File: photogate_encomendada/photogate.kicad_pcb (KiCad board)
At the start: 2 copper layers, 77.9 x 64.8 mm, 23 parts, among them P2 3poles LOGO

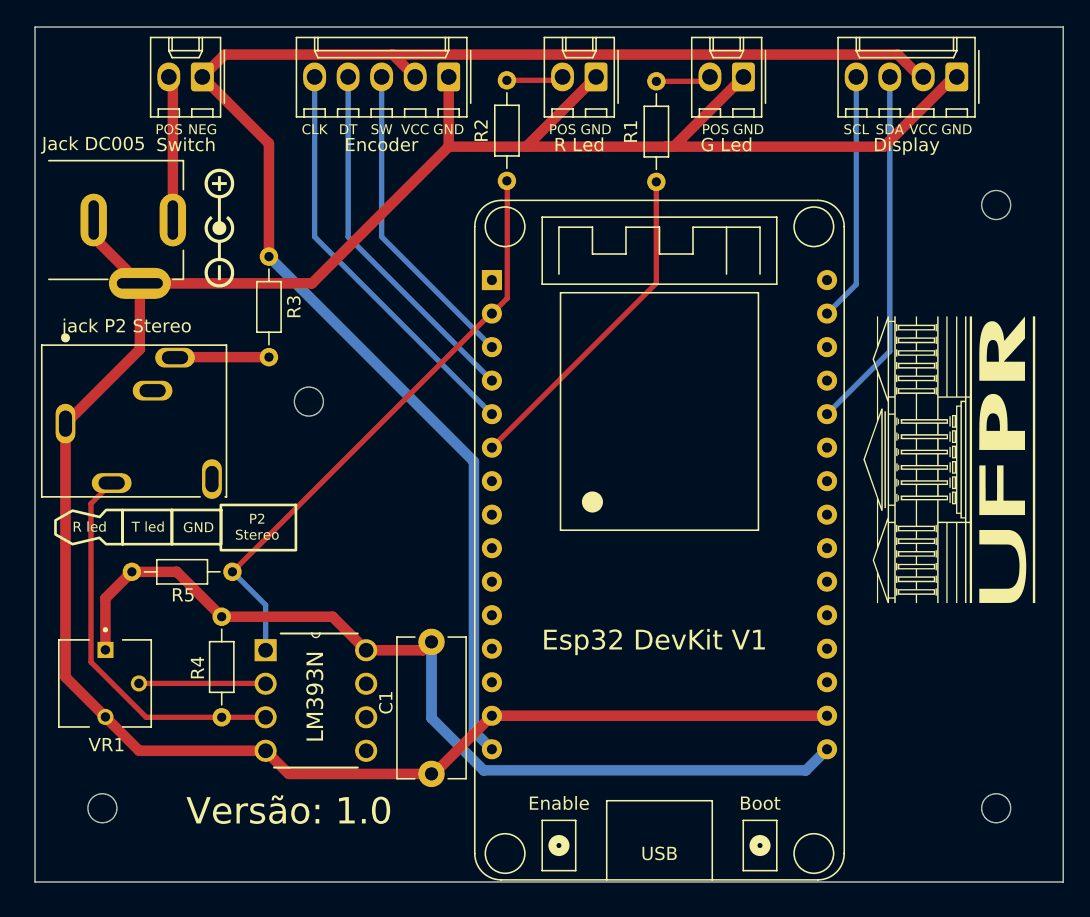
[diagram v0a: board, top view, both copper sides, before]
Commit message: Placas de fenolite e perfurada acabadas
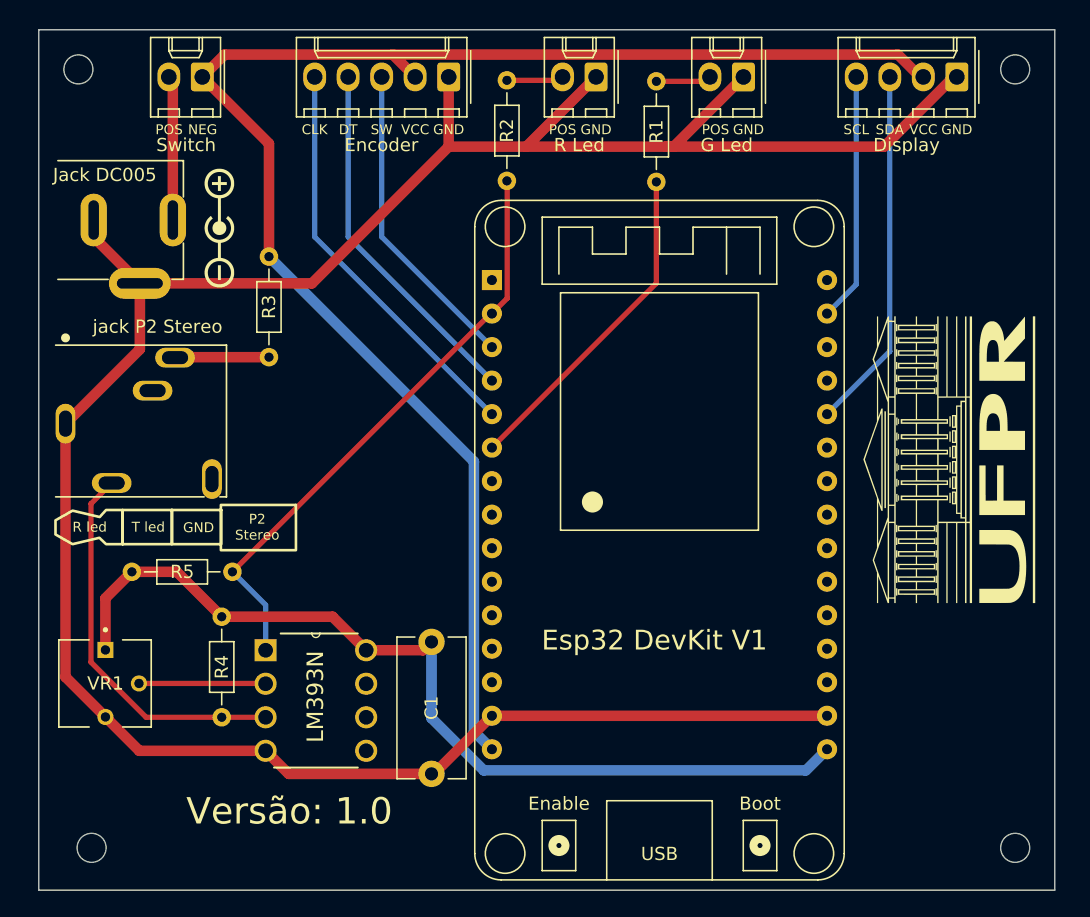
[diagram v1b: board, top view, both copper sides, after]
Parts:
- moved Furo Central 30.6 mm to (93.0, 71.0)
- moved Furo Superior 10.4 mm to (164.0, 71.0)
- moved Furo Inferior2 3.33 mm to (164.0, 130.0)
- moved Furo Inferior1 3.11 mm to (94.0, 130.0)
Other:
- board size 77.9 x 64.8 mm -> 77 x 65.2 mm
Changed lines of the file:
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@@
     (property "Sheetname" "")
     (attr through_hole)
-    (fp_text reference "jack P2 Stereo" (at 4.651 -7.3875 180) (layer "F.SilkS")
+    (fp_text reference "jack P2 Stereo" (at 6.9772 -7.3509) (layer "F.SilkS")
       (effects (font (size 1 1) (thickness 0.15)))
     )
@@
       (effects (font (size 1.401937 1.401937) (thickness 0.15)))
     )
-    (fp_line (start 10.2 5.55) (end -1.8 5.55) (layer "F.SilkS") (width 0.127))
-    (fp_line (start -1.8 5.55) (end -1.8 -5.95) (layer "F.SilkS") (width 0.127))
-    (fp_line (start -1.8 -5.95) (end 12.2 -5.95) (layer "F.SilkS") (width 0.127))
-    (fp_line (start 12.2 5.55) (end 12.1 5.55) (layer "F.SilkS") (width 0.127))
+    (fp_line (start -0.75 -5.95) (end 12.2 -5.95) (layer "F.SilkS") (width 0.127))
+    (fp_line (start 12.2 5.55) (end 11.7 5.55) (layer "F.SilkS") (width 0.127))
+    (fp_line (start -0.75 5.55) (end 10.5 5.55) (layer "F.SilkS") (width 0.127))
     (fp_line (start 12.2 -5.95) (end 12.2 5.55) (layer "F.SilkS") (width 0.127))
     (fp_circle (center 0 -6.5) (end 0.17 -6.5) (layer "F.SilkS") (width 0.34) (fill none))
@@
     (fp_line (start -5.6 3.3) (end -2.1 3.3) (layer "F.CrtYd") (width 0.05))
     (fp_line (start -5.6 -3.3) (end -5.6 3.3) (layer "F.CrtYd") (width 0.05))
-    (fp_line (start -1.8 -5.95) (end -1.8 -3) (layer "F.Fab") (width 0.127))
+    (fp_line (start -1.8 5.55) (end -1.8 -5.95) (layer "F.Fab") (width 0.127))
     (fp_line (start -5.3 -3) (end -5.3 3) (layer "F.Fab") (width 0.127))
     (fp_line (start -1.8 -3) (end -5.3 -3) (layer "F.Fab") (width 0.127))
@@
     (pad "5" thru_hole oval (at 6.6 -2.5) (size 3.016 1.508) (drill oval 2 1) (layers *.Cu *.Mask)
       (net 32 "unconnected-(P2jack1-Pad5)") (pintype "passive"))
-    (model "/home/cold/.local/share/kicad/6.0/footprints/MyFootprints.pretty/CUI_DEVICES_SJ1-3515N.step"
+    (model "/home/cold/.local/share/kicad/6.0/footprints/MyJacks.pretty/CUI_DEVICES_SJ1-3515N.step"
       (offset (xyz -5.3 0 2.5))
       (scale (xyz 1 1 1))
@@
     (property "Sheetname" "")
     (attr through_hole)
-    (fp_text reference "VR1" (at 4.6736 -0.1016 180) (layer "F.SilkS")
+    (fp_text reference "VR1" (at 0 0 180) (layer "F.SilkS")
       (effects (font (size 1.002756 1.002756) (thickness 0.15)))
     )
@@
     (pad "3" thru_hole circle (at 2.54 0 270) (size 1.222 1.222) (drill 0.714) (layers *.Cu *.Mask)
       (net 2 "GND") (pintype "passive"))
-    (model "/home/cold/.local/share/kicad/6.0/footprints/MyFootprints.pretty/TRIM_3362P-1-103.step"
+    (model "/home/cold/.local/share/kicad/6.0/footprints/trimpot.pretty/3362P-1-102.STEP"
       (offset (xyz 0 0 0))
       (scale (xyz 1 1 1))
@@
       )
     )
-    (model "/home/cold/.local/share/kicad/6.0/footprints/MyFootprints.pretty/LM393N.step"
+    (model "/home/cold/.local/share/kicad/6.0/footprints/MyCIs.pretty/LM393P.STEP"
       (offset (xyz 0 0.69 -0.5))
       (scale (xyz 1 1 1))
@@
   )
   (footprint "MountingHole:MountingHole_2.2mm_M2" (layer "F.Cu")
-    (at 162.56 127)
+    (at 164 130)
     (descr "Mounting Hole 2.2mm, no annular, M2")
     (tags "mounting hole 2.2mm no annular m2")
@@
     (property "Sheetname" "")
     (attr through_hole)
-    (fp_text reference "R5" (at 3.7338 -1.778) (layer "F.SilkS")
+    (fp_text reference "R5" (at 3.81 0) (layer "F.SilkS")
       (effects (font (size 1 1) (thickness 0.15)))
     )
@@
     (property "Sheetname" "")
     (attr through_hole)
-    (fp_text reference "Jack DC005" (at -2.29 -5.7612) (layer "F.SilkS")
+    (fp_text reference "Jack DC005" (at -1.4478 -3.4184) (layer "F.SilkS")
       (effects (font (size 1 1) (thickness 0.15)))
     )
@@
       (effects (font (size 0 0) (thickness 0.15)))
     )
-    (fp_line (start 4.51 2.3) (end 4.51 4.5) (layer "F.SilkS") (width 0.127))
-    (fp_line (start -5.6896 -4.5) (end 4.51 -4.5) (layer "F.SilkS") (width 0.127))
-    (fp_line (start 4.51 4.5) (end 3.71 4.5) (layer "F.SilkS") (width 0.127))
-    (fp_line (start -1.2192 4.5) (end -5.6896 4.5) (layer "F.SilkS") (width 0.127))
-    (fp_line (start 4.51 -4.5) (end 4.51 -2.3) (layer "F.SilkS") (width 0.127))
+    (fp_line (start 4.51 1.75) (end 4.51 4.5) (layer "F.SilkS") (width 0.127))
+    (fp_line (start 3.65 4.5) (end 4.51 4.5) (layer "F.SilkS") (width 0.127))
+    (fp_line (start -5 -4.5) (end 4.51 -4.5) (layer "F.SilkS") (width 0.127))
+    (fp_line (start -5 4.5) (end -1.2 4.5) (layer "F.SilkS") (width 0.127))
+    (fp_line (start 4.51 -4.5) (end 4.51 -1.75) (layer "F.SilkS") (width 0.127))
     (fp_line (start 4.96 -4.75) (end 4.96 6.23) (layer "F.CrtYd") (width 0.05))
     (fp_line (start -5.94 -4.75) (end 4.96 -4.75) (layer "F.CrtYd") (width 0.05))
@@
     (fp_line (start -5.94 6.23) (end -5.94 -4.75) (layer "F.CrtYd") (width 0.05))
     (fp_line (start 4.51 -4.5) (end 4.51 4.5) (layer "F.Fab") (width 0.127))
-    (fp_line (start 4.61 4.5) (end -9.69 4.5) (layer "F.Fab") (width 0.127))
+    (fp_line (start 4.51 4.5) (end -9.69 4.5) (layer "F.Fab") (width 0.127))
     (fp_line (start -9.69 4.5) (end -9.69 -4.5) (layer "F.Fab") (width 0.127))
     (fp_line (start -9.69 -4.5) (end 4.51 -4.5) (layer "F.Fab") (width 0.127))
@@
     (pad "4" thru_hole oval (at 3.71 0) (size 2 4) (drill oval 0.8 3) (layers *.Cu *.Mask)
       (net 35 "Net-(Jack_5V1-Pad4)") (pintype "passive"))
-    (model "/home/cold/.local/share/kicad/6.0/footprints/MyFootprints.pretty/NINIGI_DC-005.step"
+    (model "/home/cold/.local/share/kicad/6.0/footprints/MyJacks.pretty/DC-005.step"
       (offset (xyz -2.75 0 0))
       (scale (xyz 1 1 1))
@@
   )
   (footprint "MountingHole:MountingHole_2.2mm_M2" (layer "F.Cu")
-    (at 162.56 81.28)
+    (at 164 71)
     (descr "Mounting Hole 2.2mm, no annular, M2")
     (tags "mounting hole 2.2mm no annular m2")
@@
     (property "Sheetname" "")
     (attr through_hole)
-    (fp_text reference "R4" (at 3.8862 1.8034 90) (layer "F.SilkS")
+    (fp_text reference "R4" (at 3.81 0 90) (layer "F.SilkS")
       (effects (font (size 1 1) (thickness 0.15)))
     )
@@
   )
   (footprint "MountingHole:MountingHole_2.2mm_M2" (layer "F.Cu")
-    (at 110.4678 96.1784)
+    (at 93 71)
     (descr "Mounting Hole 2.2mm, no annular, M2")
     (tags "mounting hole 2.2mm no annular m2")
@@
     (property "Sheetname" "")
     (attr through_hole)
-    (fp_text reference "R3" (at 3.81 -1.92 90) (layer "F.SilkS")
+    (fp_text reference "R3" (at 3.81 0 90) (layer "F.SilkS")
       (effects (font (size 1 1) (thickness 0.15)))
     )
@@
     (property "Sheetname" "")
     (attr through_hole)
-    (fp_text reference "C1" (at 4.5936 3.429 -90) (layer "F.SilkS")
+    (fp_text reference "C1" (at 5 0 -90) (layer "F.SilkS")
       (effects (font (size 1 1) (thickness 0.15)))
     )
@@
     (property "Sheetname" "")
     (attr through_hole)
-    (fp_text reference "R2" (at 3.81 -1.92 90) (layer "F.SilkS")
+    (fp_text reference "R2" (at 3.81 0 90) (layer "F.SilkS")
       (effects (font (size 1 1) (thickness 0.15)))
     )
@@
     (property "Sheetname" "")
     (attr through_hole)
-    (fp_text reference "R1" (at 3.81 -1.92 90) (layer "F.SilkS")
+    (fp_text reference "R1" (at 3.81 0 90) (layer "F.SilkS")
       (effects (font (size 1 1) (thickness 0.15)))
     )
@@
   )
   (footprint "MountingHole:MountingHole_2.2mm_M2" (layer "F.Cu")
-    (at 94.82 127)
+    (at 94 130)
     (descr "Mounting Hole 2.2mm, no annular, M2")
     (tags "mounting hole 2.2mm no annular m2")
@@
       ) (layer "F.SilkS") (width 0.2) (fill none))
   )
-  (gr_rect (start 89.7128 67.7926) (end 167.64 132.588) (layer "Edge.Cuts") (width 0.1) (fill none))
+  (gr_rect (start 90 68) (end 167 133.2074) (layer "Edge.Cuts") (width 0.1) (fill none))
   (gr_text "Feito por: \nMarcio Ap. Bulla Jr.\n\nOrientado pelo:\nFabiano Yokaichiya\n\nCódigo Fonte: \ngithub.com/MarcioBulla/Cronometro-Optico\n" (at 137.1346 81.1022 90) (layer "B.SilkS")
     (effects (font (size 1.5 1.5) (thickness 0.3) italic) (justify left mirror))
